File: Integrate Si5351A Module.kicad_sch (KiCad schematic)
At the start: 7 parts, among them J1 DC-005-5A-2.0, J2 TYPE-C-31-M-12, U1 USBLC6-2SC6

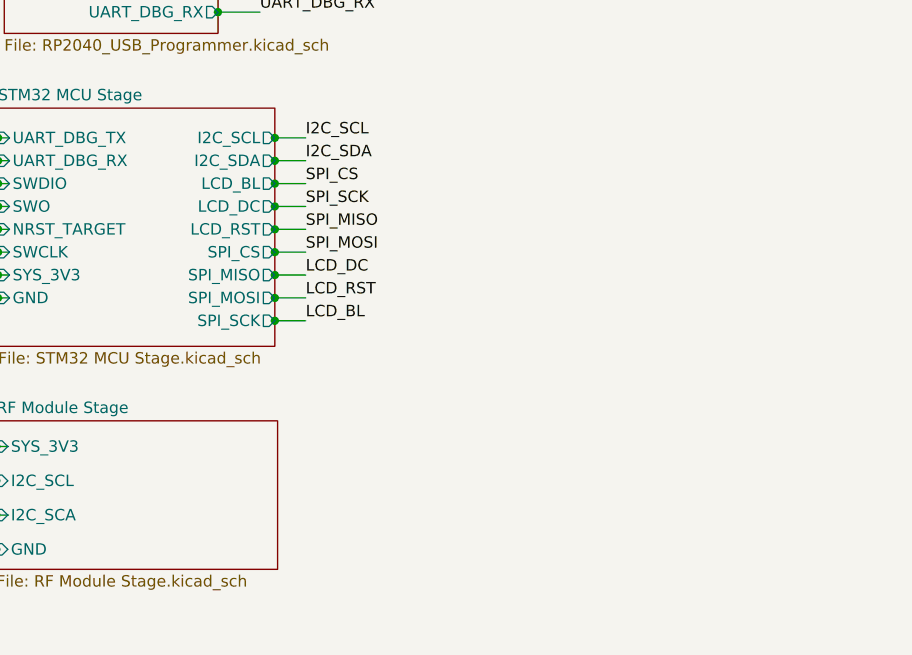
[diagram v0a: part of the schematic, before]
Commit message: LCD Stage Finished
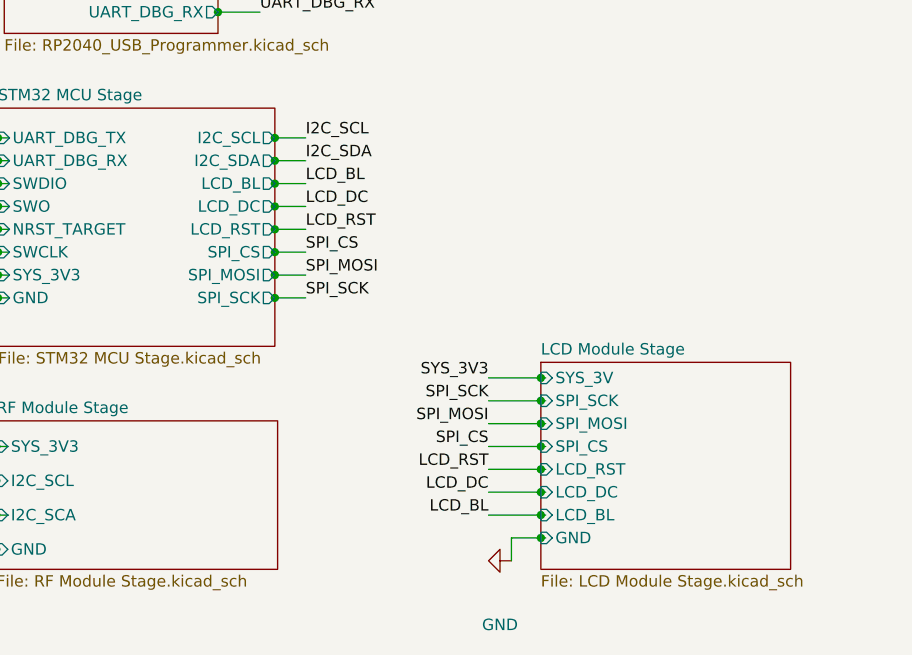
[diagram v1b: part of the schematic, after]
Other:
- added sheet LCD Module Stage (LCD Module Stage.kicad_sch)
- sheet STM32 MCU Stage ports: added none; removed SPI_MISO
